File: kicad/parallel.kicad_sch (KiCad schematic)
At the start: 17 parts, among them J8 LPT_IDC, U143 74LS244, U152 74LS155, U153 74LS367, U166 74LS05, U167 74LS174, U168 74LS240, U169 74LS374, U175 74LS04

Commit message: Add parallel port, game port
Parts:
- removed unit 4 of U175
- removed unit 5 of U175
- added C81: C_Small, seequa_footprints:C_Seequa_Bypass_6.5mm, symbol Device:C_Small
- added RN13: R_Network05_Split, Resistor_THT:R_Array_SIP6, symbol Device:R_Network05_Split
- U153: seq_notes LPT Status Register -> LPT Read Register 0
- U167: seq_notes LPT Control Register -> LPT Control Write Register
- U168: seq_notes (none) -> LPT Read Register 1
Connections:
- net C_IRQ_{EN} is gone; now on net LPT_IRQ_EN: U167.15 (Q5)
- net S_ERROR is gone; now on net ~{ERR}: U153.12 (I5)
- net ~{LPT_DATA_{CS}} is gone; now on net ~{LPT_DATA_{RD}}: U143.19 (OEb), U152.7 (Q0a)
- net ~{LPT_STATUS_{CS2}} is gone; now on net ~{LPT_CONTROL_{RD}}: U152.5 (Q2a), U153.1 (OEa)
- net +5V: now also U166.14 (VCC), U175.14 (VCC), RN13.1 (R1), RN13.1 (R1), RN13.1 (R1), RN13.1 (R1), RN13.1 (R1)
- net BUSY: no longer U168.8 (I3a)
- net GND: now also U166.7 (GND), U169.1 (OE), U175.7 (GND), C81.2
- net LPT_SELECT_IN: no longer U168.3 (O3b), U169.8 (D3)
- net PD0: now also U143.9 (O0b), U168.3 (O3b), U169.8 (D3)
- net PD1: now also U143.3 (O3b), U169.18 (D7)
- net PD2: now also U143.14 (O2a), U169.7 (D2); no longer U168.16 (O1a)
- net PD3: now also U143.16 (O1a), U169.17 (D6)
- net PD4: now also U143.5 (O2b), U169.4 (D1)
- net PD5: now also U143.7 (O1b), U168.16 (O1a), U169.14 (D5)
- net PD6: now also U143.18 (O0a), U169.3 (D0)
- net PD7: now also U143.12 (O3a), U169.13 (D4)
- net PE: now also U175.3
- net SELECT: now also U175.5
- net ~{AFD}: now also U168.13 (I1b), RN13.4 (R3.2)
- net ~{INIT}: now also U166.13, RN13.2 (R1.2)
- net ~{SELECT_IN}: now also U168.11 (I0b)
- net ~{STB}: now also U168.17 (I3b), C81.1, RN13.5 (R4.2)
- net LD3: now reaches C76.1, J8.9 (PD3)
- net LD3: now also U143.4 (I1a), U169.16 (O6)
- net LD1: now reaches C74.1, J8.5 (PD1)
- net LD1: now also U143.17 (I3b), U169.19 (O7)
- net LD2: now reaches C75.1, J8.7 (PD2)
- net LD2: now also U143.6 (I2a), U169.6 (O2)
- net LPT_IRQ_EN: now reaches U153.10 (I4)
- net INT: now reaches U153.6 (I3)
- net S_PE: now reaches U175.4
- net S_PE: now also U168.4 (I1a)
- net S_SELECT: now reaches U175.6
- net S_SELECT: now also U168.2 (I0a)
- net ~{LPT_DATA_{WR}}: now reaches U152.9 (Q0b)
- net ~{LPT_DATA_{WR}}: now also U169.11 (Cp)
- net INIT': now reaches U166.1, U166.8
- net INIT': now also RN13.6 (R5.2)
- net LD7: now reaches C80.2, J8.17 (PD7)
- net LD7: now also U143.8 (I3a), U169.12 (O4)
- net LD5: now reaches U169.15 (O5)
- net LD5: now also C78.1, J8.13 (PD5), U143.13 (I1b)
- net LD6: now reaches U169.2 (O0)
- net LD6: now also C79.1, J8.15 (PD6), U143.2 (I0a)
- net LD4: now reaches U143.15 (I2b), U169.5 (O1)
- net LD4: now also C77.1, J8.11 (PD4)
- net LD0: now reaches U169.9 (O3)
- net LD0: now also C73.1, J8.3 (PD0), U143.11 (I0b)
- net INIT: now reaches U168.15 (I2b)
- net INIT: now also U166.12, RN13.3 (R2.2)
- net ~{LPT_CONTROL_{RD}}: now reaches U168.19 (OEb)
- net ~{S_ACK}: now reaches U168.6 (I2a)
- net ~{LPT_DATA_{RD}}: now reaches U143.1 (OEa)
- net C_SELECT renamed C_SELECT_IN
- net LPT_IRQACK renamed LPT_ACK
- net ~{LPT_CONTROL_{CS}} renamed ~{LPT_CONTROL_{WR}}
- net ~{LPT_S_ACK} renamed ~{IO_NMI}
- new net ~{S_BUSY}: U168.8 (I3a)
- no-connect marks 0 -> 2
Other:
- note added: "LPT Control Register - 37Eh"
- note added: "LPT Status Register - 37Dh"
- note added: "To NMI control PAL (page 2)"
- note added: "To Parallel Port"
- note added: "To U168 Control Readback Register"
- title: (none) -> Parallel Port
- moved on the sheet: C73, C74, C75, C76, C77, C78, C79, C80, J8, U143, U166A, U166B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

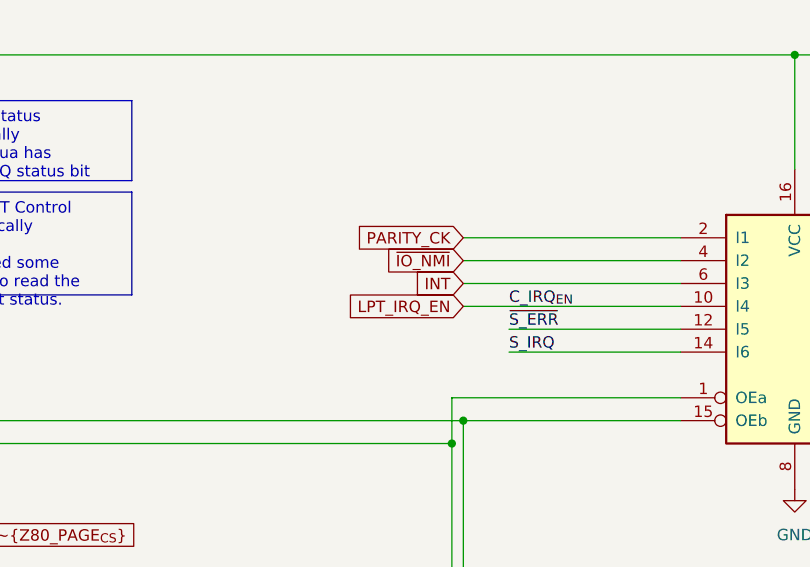
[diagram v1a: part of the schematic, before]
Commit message: Updates, chameleon logo
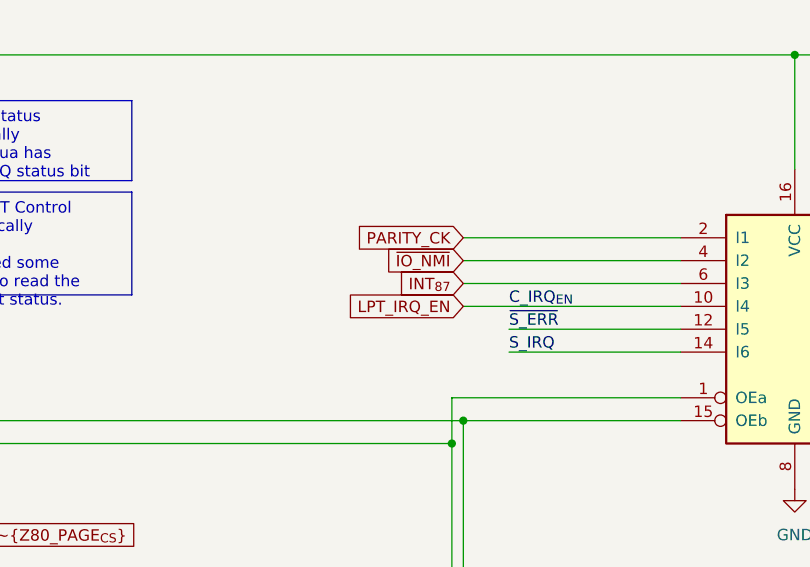
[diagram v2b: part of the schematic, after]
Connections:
- net INT renamed INT_{87}
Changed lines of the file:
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@@
 		)
 	)
-	(global_label "INT"
+	(global_label "INT_{87}"
 		(shape input)
 		(at 170.18 41.91 180)
